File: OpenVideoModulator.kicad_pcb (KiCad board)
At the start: 2 copper layers, 32 x 25 mm, 22 parts, among them J1 CONN_6, J2 Conn_Coaxial, P1 OSHW_LOGO, U1 AD724, Y1 4.433619M

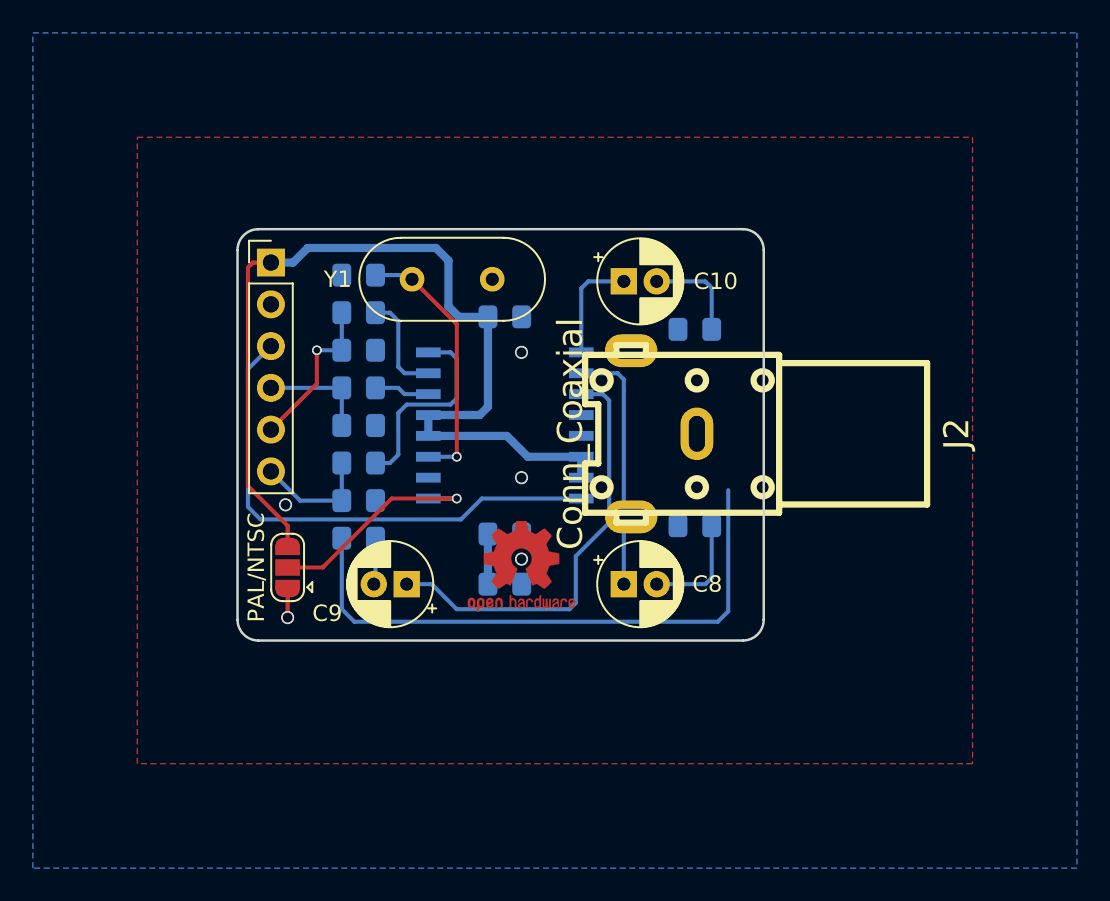
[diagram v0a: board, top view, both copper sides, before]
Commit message: Almost there...
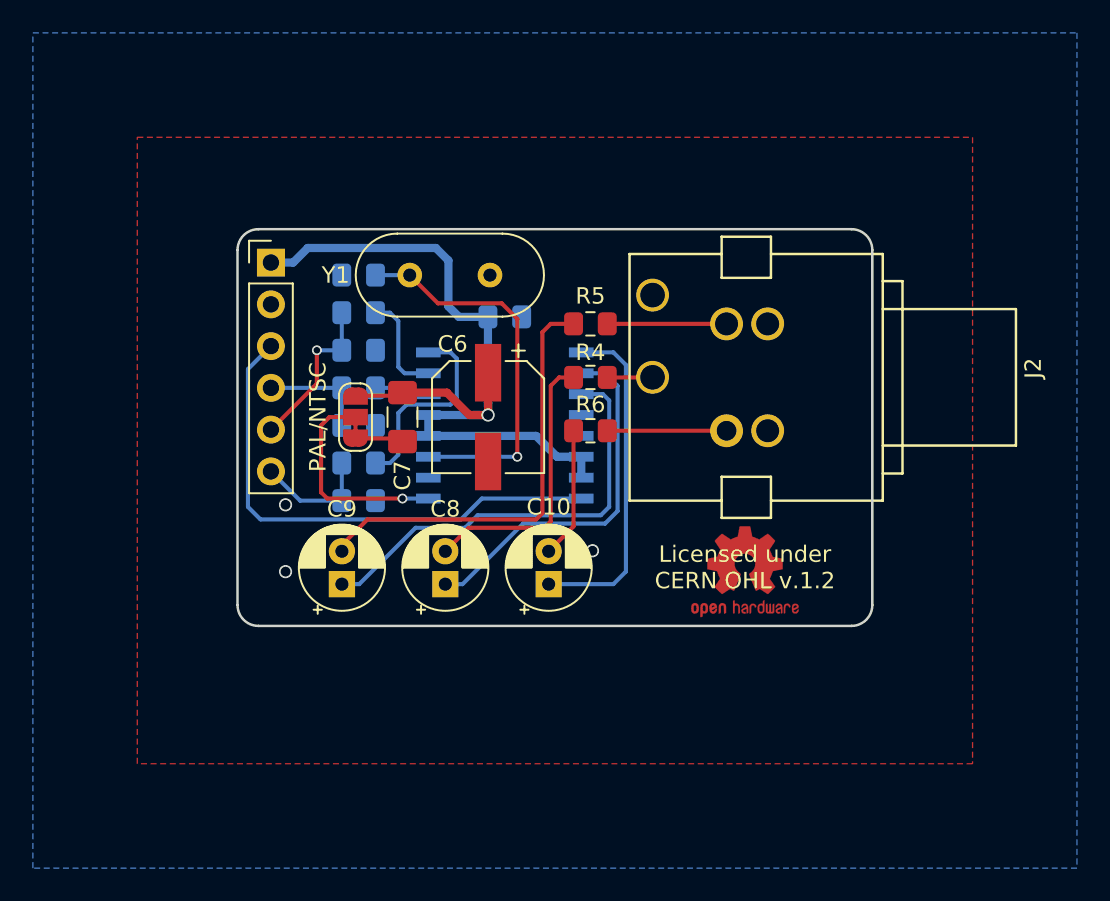
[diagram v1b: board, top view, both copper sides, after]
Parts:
- C6: footprint Capacitor_SMD:C_0805_2012Metric_Pad1.15x1.40mm_HandSolder -> Capacitor_SMD:CP_Elec_6.3x5.8; moved to F.Cu
- C7: footprint Capacitor_SMD:C_0805_2012Metric_Pad1.15x1.40mm_HandSolder -> Capacitor_SMD:C_1206_3216Metric_Pad1.42x1.75mm_HandSolder; moved to F.Cu
- J2: value Conn_Coaxial -> S-Video+Composite_Combo; footprint w_conn_av:rca_yellow -> OpenVideoModulator:AV-MDC-401
- JP1: footprint Jumper:SolderJumper-3_P1.3mm_Open_RoundedPad1.0x1.5mm -> OpenVideoModulator:SolderJumper-3_P1.3mm_Bridged12_RoundedPad1.0x1.5mm
- R4, R5, R6: moved to F.Cu
- Y1: footprint Crystal:Crystal_HC49-U_Vertical -> Crystal:Crystal_HC49-4H_Vertical
- moved R5 19.2 mm to (135.5, 55.8), turned to 180 degrees
- moved C10 19.0 mm to (133.0, 71.6), turned to 90 degrees
- moved P1 13.6 mm to (144.9, 70.9)
- moved J2 12.0 mm to (153.3, 66.5)
- moved R4 11.0 mm to (135.5, 59.1), turned to 180 degrees
- moved C8 10.9 mm to (126.7, 71.6), turned to 90 degrees
- moved C6 10.2 mm to (129.3, 61.5), turned to 270 degrees
- moved JP1 10.0 mm to (121.2, 61.5)
- moved C7 9.45 mm to (124.1, 61.5), turned to 90 degrees
- moved R6 8.85 mm to (135.5, 62.3), turned to 180 degrees
- moved C9 3.94 mm to (120.4, 71.6), turned to 90 degrees
- moved Y1 0.29 mm to (129.4, 52.8)
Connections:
- C5 pad 2: VCC -> VAA
- J1 pad 1: VCC -> VAA
- J2 pad 1: Net-(J2-Pad1) -> GND
- JP1 pad 3: VCC -> VAA
- R4 pad 1: Net-(J2-Pad1) -> Net-(J2-Pad6)
- R5 pad 1: Net-(J3-Pad3) -> Net-(J2-Pad3)
- R6 pad 1: Net-(J3-Pad4) -> Net-(J2-Pad4)
- U1 pad 14: VCC -> VAA
- U1 pad 15: VCC -> VAA
- U1 pad 4: VCC -> VAA
- U1 pad 5: VCC -> VAA
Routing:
- net VCC: track 58.1 -> 0.00 mm
- net VAA: track 3.05 -> 50.8 mm, vias 0 -> 1
- net Net-(J3-Pad3): track 35.8 -> 0.00 mm
- net Net-(C9-Pad2): track 2.90 -> 26.1 mm
- net Net-(C10-Pad1): track 6.66 -> 20.6 mm
- net Net-(C8-Pad2): track 6.68 -> 17.0 mm
- net Net-(C1-Pad1): track 16.0 -> 23.9 mm
- net Net-(C8-Pad1): track 15.2 -> 22.5 mm
- net Net-(J2-Pad4): track 0.00 -> 7.25 mm
- net Net-(J2-Pad3): track 0.00 -> 7.25 mm
- net Net-(J2-Pad6): track 0.00 -> 2.76 mm
- net Net-(C10-Pad2): track 6.04 -> 8.30 mm
- net GND: track 1.75 -> 2.94 mm, vias 5 -> 3
- net Net-(JP1-Pad2): track 13.8 -> 13.1 mm
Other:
- board size 32 x 25 mm -> 38.6 x 24.1 mm
- rule pad_to_mask_clearance: 0.051 -> 0
- rule solder_mask_min_width: 0.25 -> 0.2
- board text added: "Licensed under CERN OHL v.1.2"
- board text added: "V1"
